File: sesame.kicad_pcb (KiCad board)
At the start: 2 copper layers, 169 parts, among them U1 ATmega32A-PU

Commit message: Add files via upload
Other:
- board outline added: 370.3 x 130.8 mm

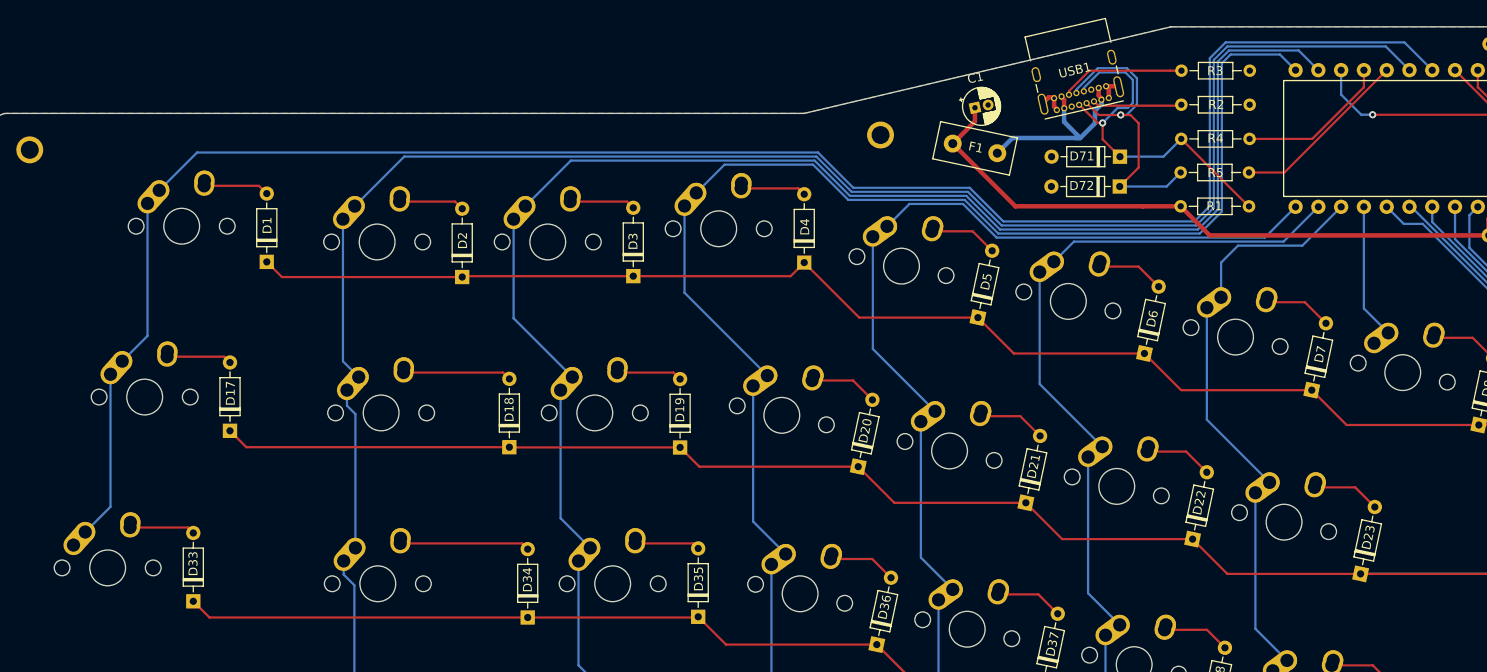
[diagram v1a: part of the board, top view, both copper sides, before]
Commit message: Add files via upload
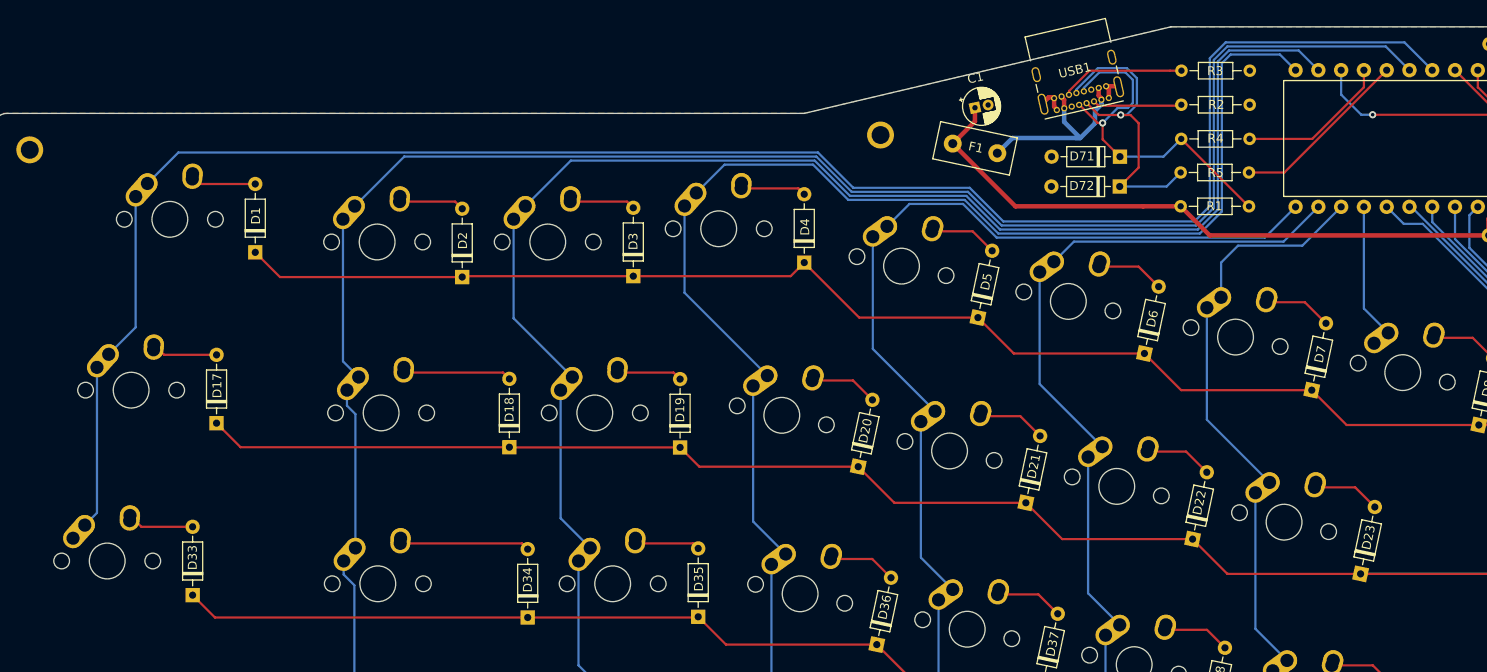
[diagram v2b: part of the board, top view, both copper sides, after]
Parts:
- moved D17 1.72 mm to (46.0, 107.7)
- moved MX17 1.70 mm to (36.4, 104.0)
- moved D1 1.67 mm to (50.3, 88.6)
- moved MX1 1.53 mm to (40.8, 85.0)
- moved MX33 0.77 mm to (33.8, 123.1)
- moved D33 0.69 mm to (43.3, 126.9)
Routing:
- net row1: track 409.8 -> 411.7 mm
- net row0: track 378.4 -> 380.2 mm
- net Net-(D1-Pad2): track 7.94 -> 7.26 mm
